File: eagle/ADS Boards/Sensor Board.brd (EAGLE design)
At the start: 61.7 x 61.7 mm, 19 parts, among them J1 S2B-PH-SM4-TB(LF)(SN), J2 S2B-PH-SM4-TB(LF)(SN), J3 S2B-PH-SM4-TB(LF)(SN), J4 S2B-PH-SM4-TB(LF)(SN), J5 S2B-PH-SM4-TB(LF)(SN), J6 S2B-PH-SM4-TB(LF)(SN), J7 62674-121121ALF

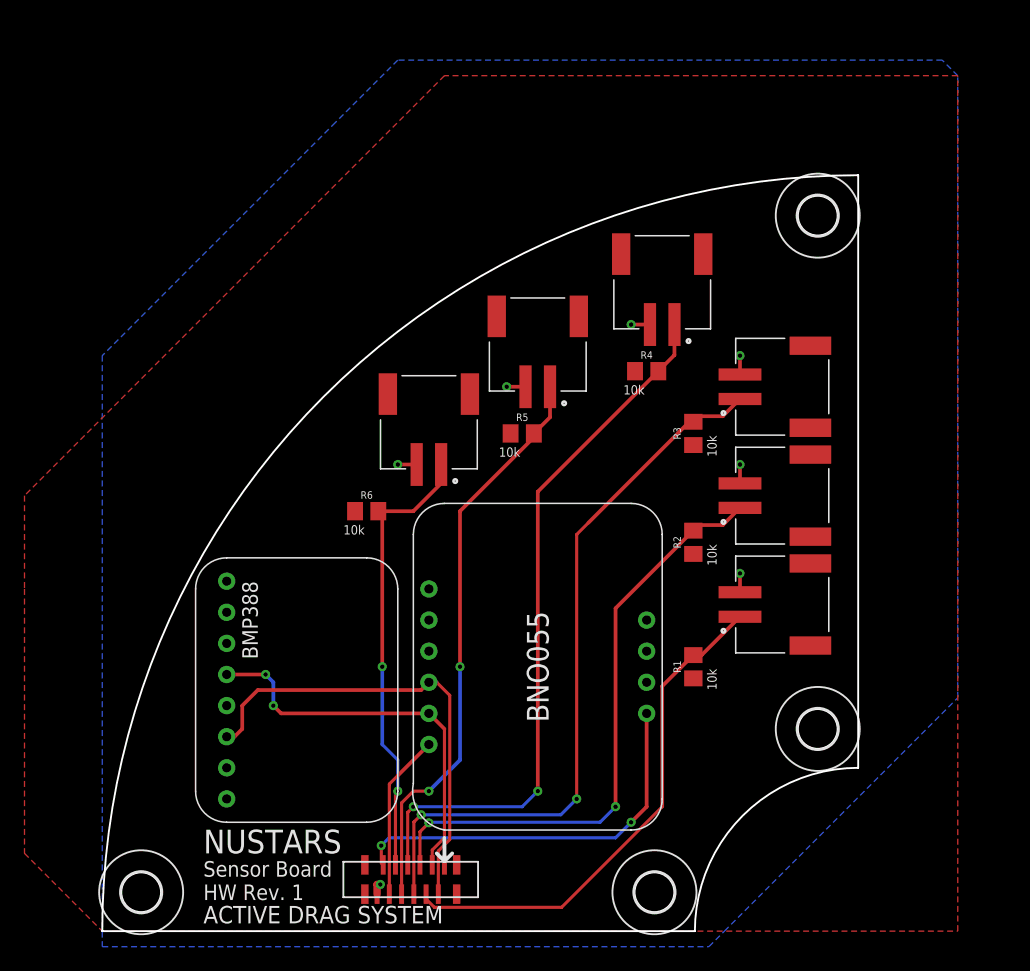
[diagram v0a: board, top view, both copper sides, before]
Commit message: fixed rocket boards
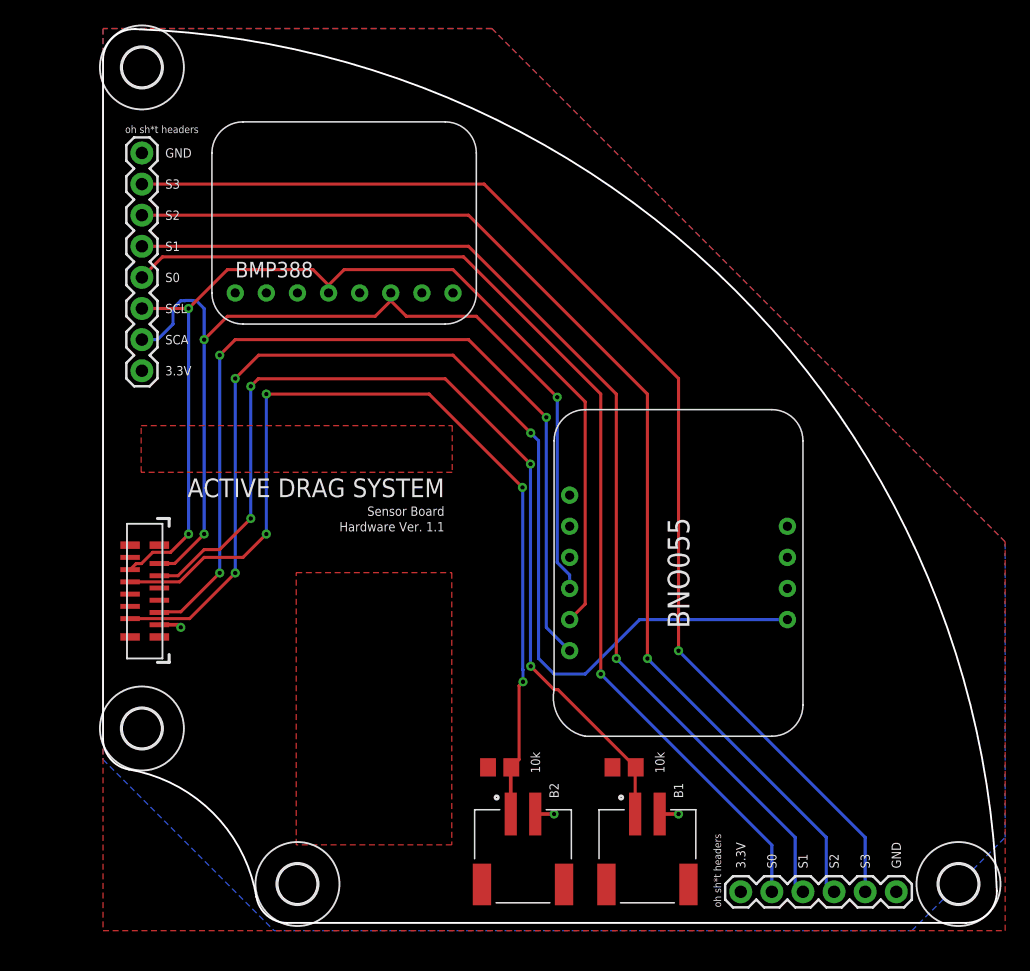
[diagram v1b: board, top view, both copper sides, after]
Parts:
- removed J5, J6: S2B-PH-SM4-TB(LF)(SN), S2B-PH-SM4-TB_LF__SN_:JST_S2B-PH-SM4-TB(LF)(SN)
- removed R3, R4, R5, R6: 10k, resistor:R0805
- J3: value S2B-PH-SM4-TB(LF)(SN) -> (none); device S2B-PH-SM4-TB_LF__SN_:JST_S2B-PH-SM4-TB(LF)(SN) -> SparkFun-Connectors:1X08
- J4: value S2B-PH-SM4-TB(LF)(SN) -> (none); device S2B-PH-SM4-TB_LF__SN_:JST_S2B-PH-SM4-TB(LF)(SN) -> SparkFun-Connectors:1X06
- moved H1 67.3 mm to (3.24, 70.5), turned to 270 degrees
- moved H4 55.8 mm to (69.9, 3.85), turned to 270 degrees
- moved J3 48.9 mm to (3.24, 45.8)
- moved J4 46.8 mm to (52.1, 3.21), turned to 0 degrees
- moved H3 44.3 mm to (15.9, 3.85)
- moved H2 43.9 mm to (3.24, 16.5), turned to 270 degrees
- moved J7 36.5 mm to (7.05, 30.5), turned to 90 degrees
- moved J2 31.5 mm to (34.4, 9.56), turned to 0 degrees
- moved R2 24.2 mm to (32.4, 13.4), turned to 0 degrees
- moved U$1 19.1 mm to (8.95, 49.6), turned to 0 degrees
- moved J1 18.7 mm to (44.5, 9.56), turned to 0 degrees
- moved U$2 13.8 mm to (36.9, 42.6)
- moved R1 9.97 mm to (42.6, 13.4), turned to 0 degrees
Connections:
- removed net B3: J3.1, J7.6, R3.2
- removed net B4: J4.1, J7.7, R4.2
- removed net B5: J5.1, J7.8, R5.2
- removed net B6: J6.1, J7.9, R6.2
- new net S0: J3.4, J4.2
- new net S1: J3.5, J4.3
- new net S2: J3.6, J4.4
- new net S3: J3.7, J4.5
- net 3.3V: now also J3.1, J4.1; no longer R3.1, R4.1, R5.1, R6.1
- net GND: now also J3.8, J4.6; no longer J3.2, J4.2, J5.2, J6.2
- net SCL: now also J3.3
- net SDA: now also J3.2
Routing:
- net S3: track 0.00 -> 98.6 mm, vias 0 -> 1
- net S2: track 0.00 -> 94.3 mm, vias 0 -> 1
- net S1: track 0.00 -> 90.7 mm, vias 0 -> 1
- net S0: track 0.00 -> 89.2 mm, vias 0 -> 1
- net ADR: track 32.2 -> 94.9 mm, vias 2 -> 3
- net RST: track 13.6 -> 73.7 mm, vias 0 -> 3
- net B3: track 59.5 -> 0.00 mm, vias 2 -> 0
- net B4: track 58.3 -> 0.00 mm, vias 2 -> 0
- net SCL: track 32.3 -> 86.4 mm
- net B5: track 47.2 -> 0.00 mm, vias 2 -> 0
- net SDA: track 38.2 -> 80.6 mm, vias 0 -> 3
- net B6: track 37.2 -> 0.00 mm, vias 2 -> 0
- net B1: track 41.9 -> 78.5 mm, vias 0 -> 4
- net B2: track 49.5 -> 75.3 mm, vias 2 -> 4
- net GND: track 10.9 -> 4.92 mm, vias 7 -> 3
- added copper zone on layer 1, net D2
- added copper zone on layer 1, net DUMMY
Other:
- board size 61.7 x 61.7 mm -> 73 x 73 mm
- board text added: "3.3V"
- board text added: "B1"
- board text added: "B2"
- board text added: "C:/Users/ichis/Pictures/Cornket.bmp"
- board text added: "C:/Users/ichis/Pictures/NUSTARS Logo PNG.bmp"
- board text added: "GND"
- board text added: "Hardware Ver. 1.1"
- board text added: "S0"
- board text added: "S1"
- board text added: "S2"
- board text added: "S3"
- board text added: "SCA"
- board text added: "SCL"
- board text added: "oh sh*t headers"
- board text removed: "HW Rev. 1"
- board text removed: "NUSTARS"
